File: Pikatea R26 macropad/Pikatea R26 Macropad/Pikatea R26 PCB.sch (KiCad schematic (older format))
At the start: 37 parts, among them J1 AVR-ISP-6, J2 USB_B_Mini, J3 Conn_01x04_Male, J4 Conn_01x04_Male, SW1 SW_DPST, SW2 Rotary_Encoder_Switch, U1 ATMEGA32U4-EP, U2 USBLC6-2P6, Y1 16MHz

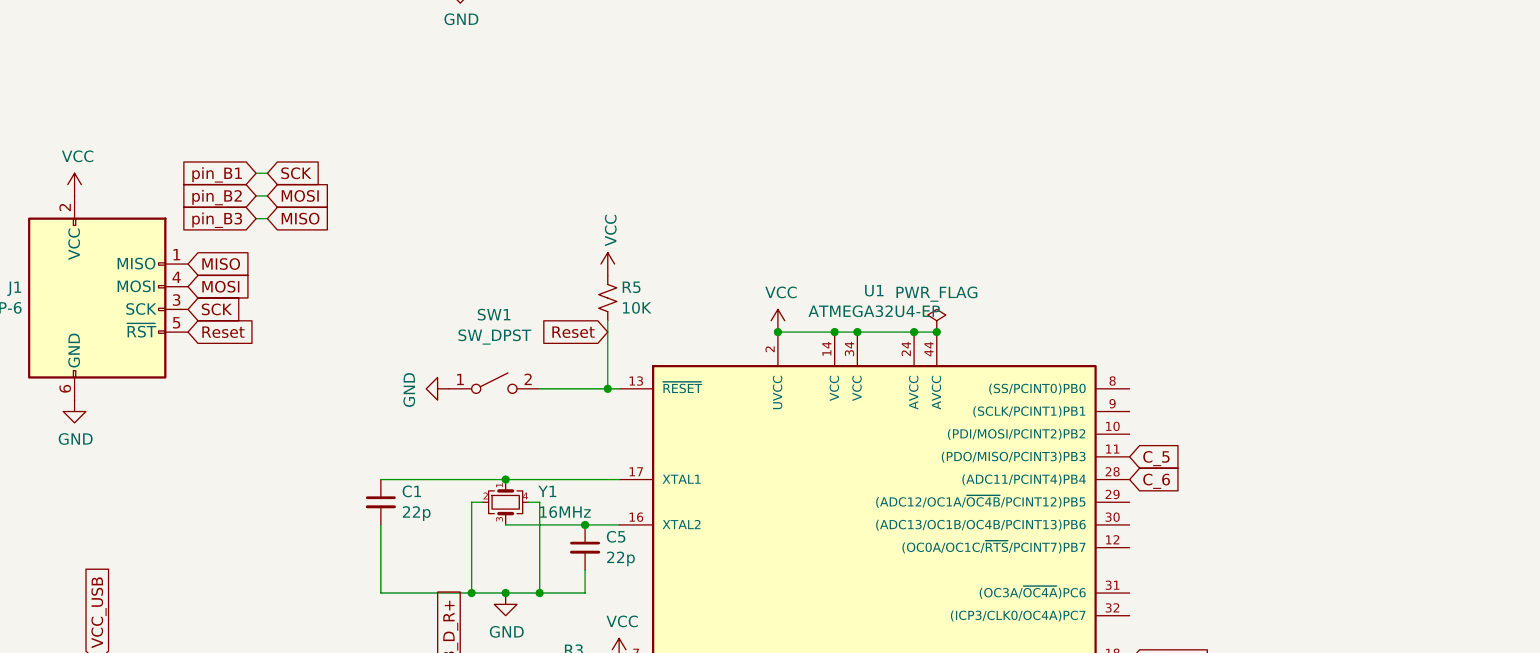
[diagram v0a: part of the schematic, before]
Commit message: update R26
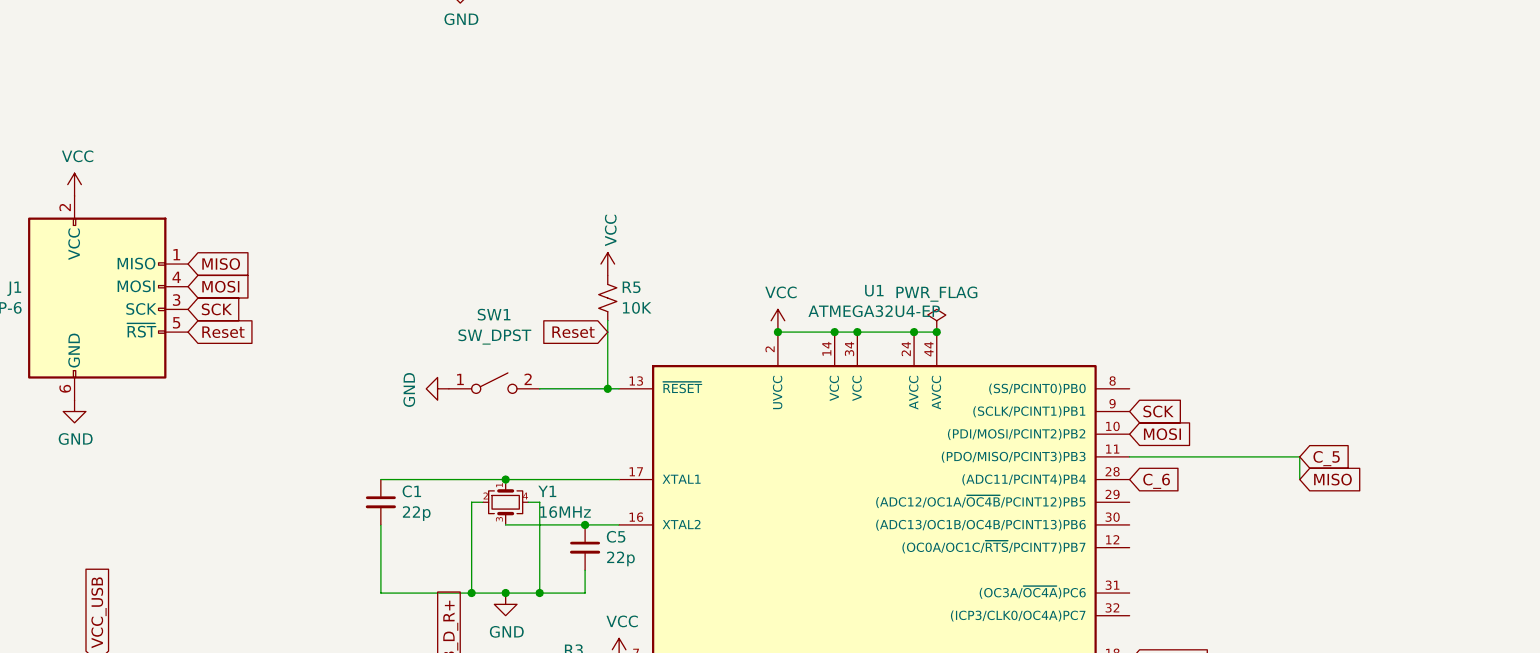
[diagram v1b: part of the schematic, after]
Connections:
- net MISO is gone; now on net C_5: J1.1 (MISO)
- net MOSI: now also U1.10 ((PDI/MOSI/PCINT2)PB2)
- net SCK: now also U1.9 ((SCLK/PCINT1)PB1)
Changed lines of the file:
@@
 Text GLabel 18450 5300 2    50   Input ~ 0
 USB_D+
-Text GLabel 19700 2600 2    50   Input ~ 0
-MOSI
-Text GLabel 19700 2700 2    50   Input ~ 0
-MISO
-Text GLabel 19650 2500 0    50   Input ~ 0
-pin_B1
-Text GLabel 19650 2600 0    50   Input ~ 0
-pin_B2
-Text GLabel 19650 2700 0    50   Input ~ 0
-pin_B3
-Text GLabel 19700 2500 2    50   Input ~ 0
-SCK
-Wire Wire Line
-	19700 2500 19650 2500
-Wire Wire Line
-	19700 2600 19650 2600
-Wire Wire Line
-	19700 2700 19650 2700
 Wire Wire Line
 	18350 5200 18550 5200
@@
 Text GLabel 23500 4750 2    50   Input ~ 0
 Knob_B
-Text GLabel 23500 3750 2    50   Input ~ 0
+Text GLabel 24250 3750 2    50   Input ~ 0
 C_5
 Text GLabel 23500 5050 2    50   Input ~ 0
@@
 Text GLabel 16800 5200 2    50   Input ~ 0
 VCC_USB
+Text GLabel 23500 3650 2    50   Input ~ 0
+MOSI
+Text GLabel 24250 3850 2    50   Input ~ 0
+MISO
+Wire Wire Line
+	24250 3850 24250 3750
+Wire Wire Line
+	23500 3750 24250 3750
+Text GLabel 23500 3550 2    50   Input ~ 0
+SCK
 $EndSCHEMATC

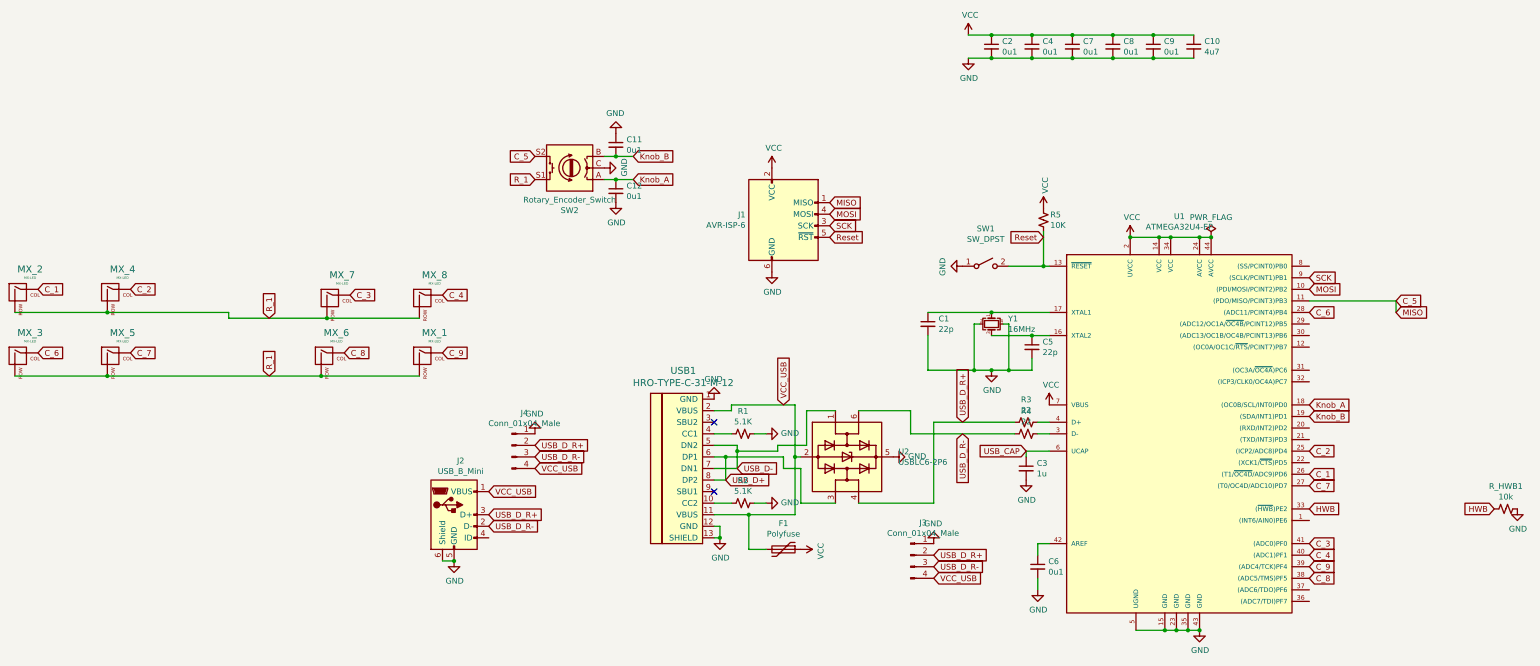
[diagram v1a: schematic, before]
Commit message: updates
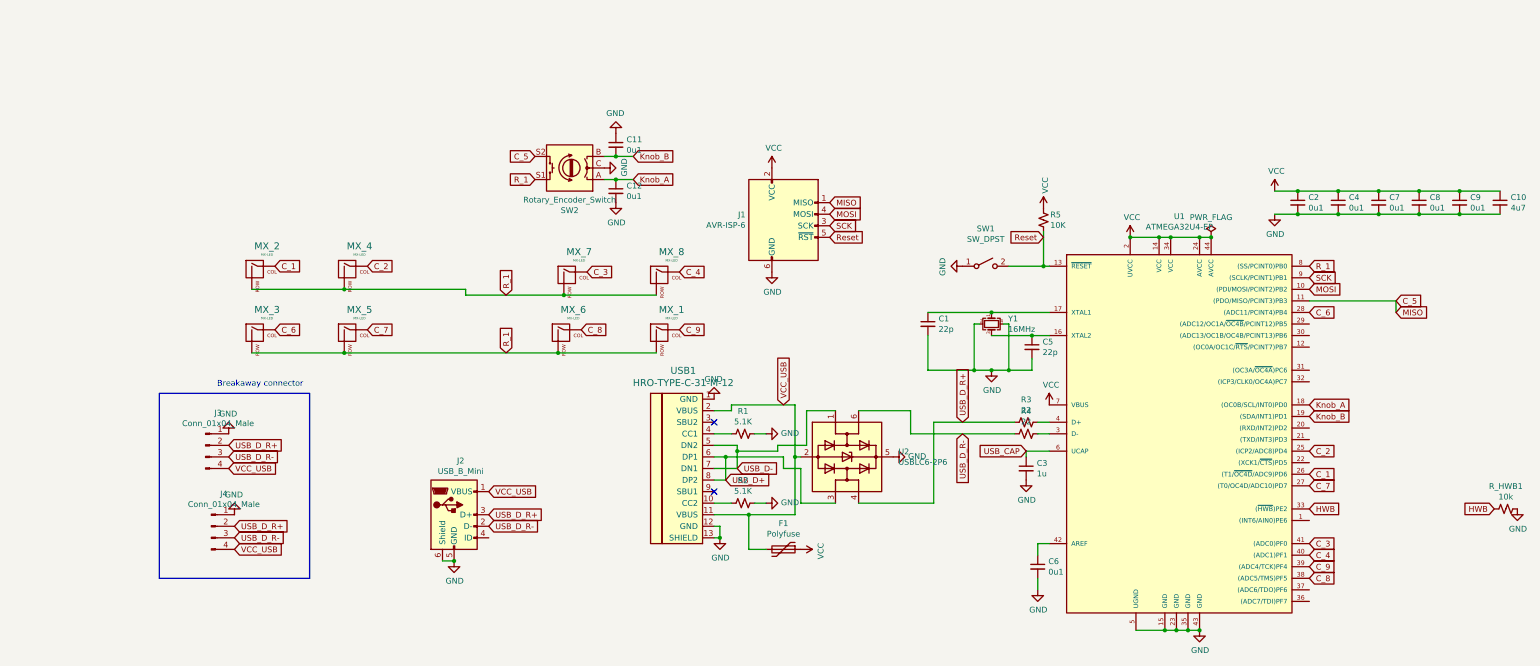
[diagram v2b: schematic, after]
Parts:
- USB1: footprint Type-C:HRO-TYPE-C-31-M-13 -> Type-C:HRO-TYPE-C-31-M-12
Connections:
- net R_1: now also U1.8 ((SS/PCINT0)PB0)
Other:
- note added: "Breakaway connector\n"
- moved on the sheet: C10, C2, C4, C7, C8, C9, J3, J4, MX_1, MX_2, MX_3, MX_4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
